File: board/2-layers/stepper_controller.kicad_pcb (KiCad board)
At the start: 4 copper layers, 99 x 46 mm, 126 parts, among them J201 USB_OTG, P101 JTAG, P102 JTAG, P103 CONN_4, P104 CONN_8X2, P105 CONN_4, P106 CONN_6X2, P107 CONN_4, P201 CONN_2X2, P301 12V_Conn, U101 DRV8825, U102 DRV8825, U103 DRV8825, U104 MAX5713/4/5-TSSOP14, U201 STM32F103RG_LQFP64, U301 MP2128-SOT23, U302 MP2303_SOIC8E, U401 XC3S200A, X201 TXC_50X32_AB

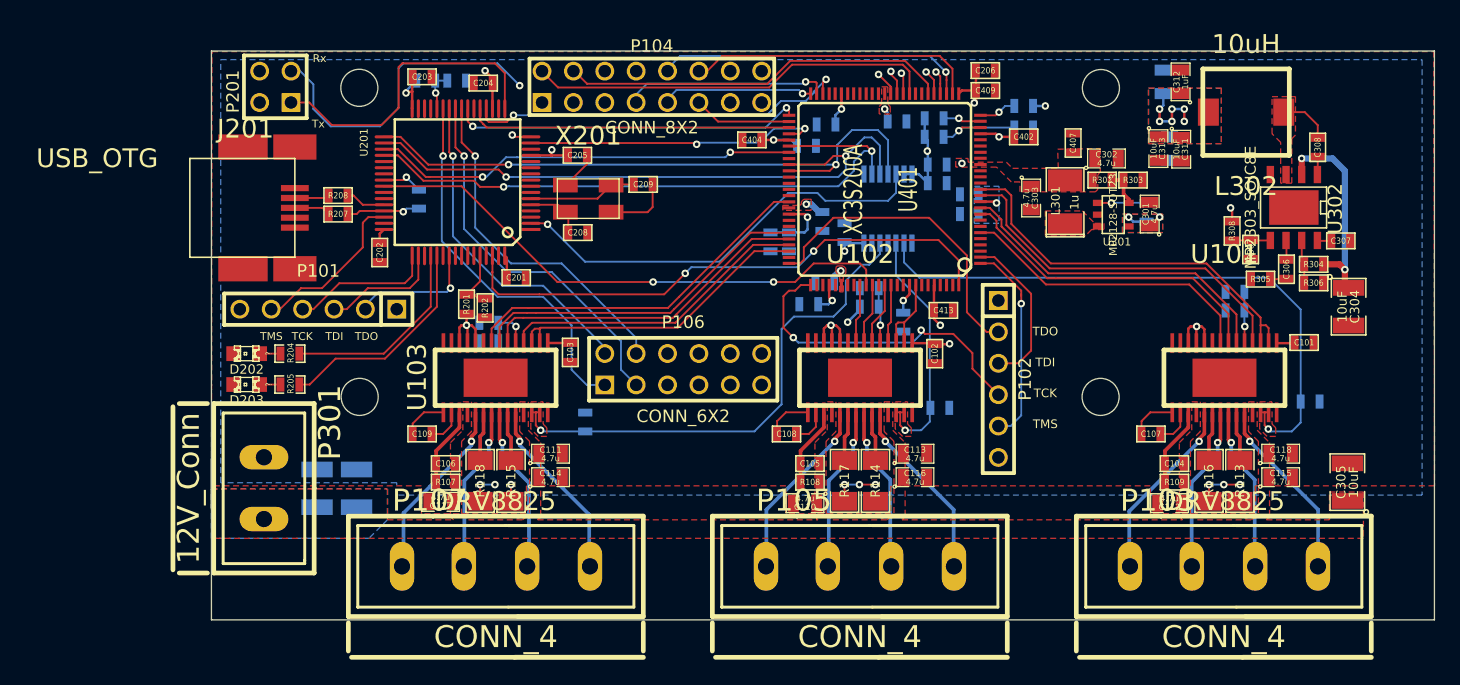
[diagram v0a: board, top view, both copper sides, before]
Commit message: pouet
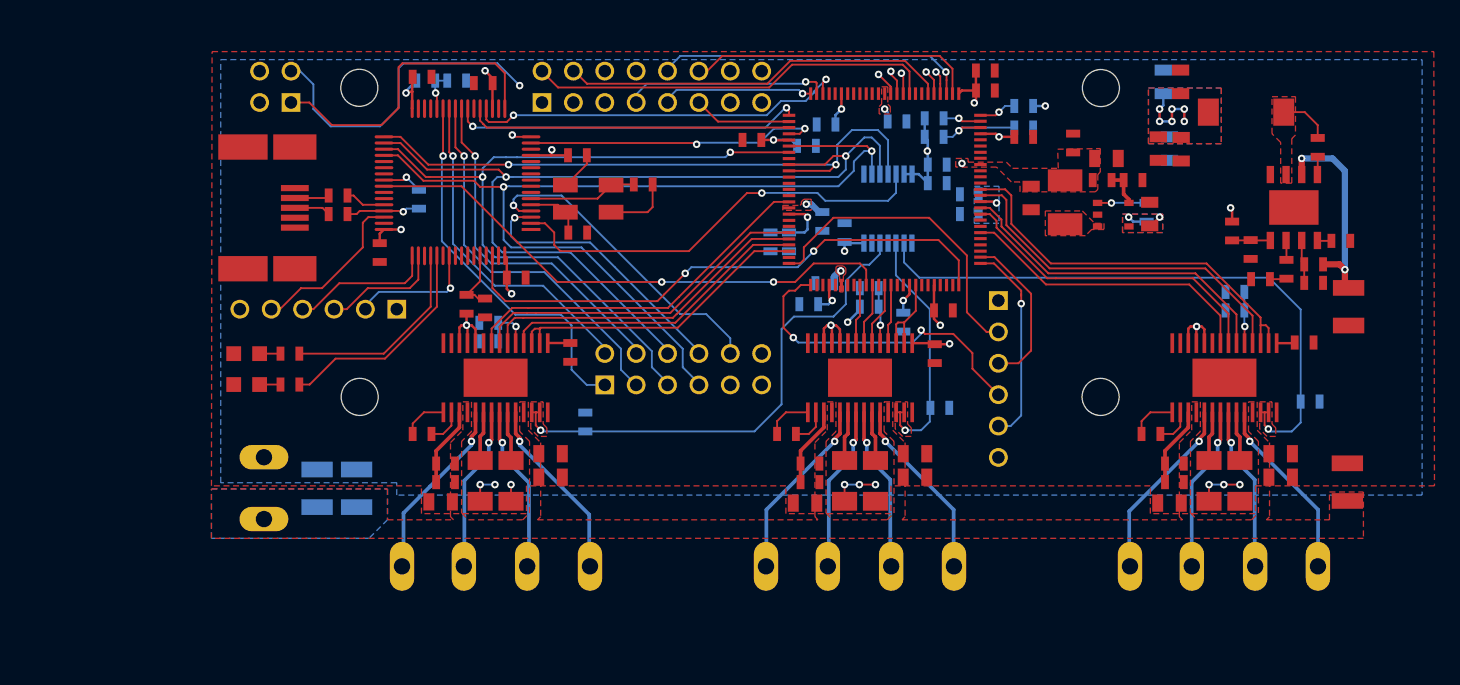
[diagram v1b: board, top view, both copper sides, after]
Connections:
- P106 pad 10: (no net) -> /STM32/PC15
- P106 pad 5: (no net) -> /FPGA/COM_MISO
- P106 pad 6: (no net) -> /FPGA/COM_CLK
- P106 pad 7: (no net) -> /FPGA/COM_MOSI
- P106 pad 8: (no net) -> /STM32/PC14
- U201 pad 3: (no net) -> /STM32/PC14
- U201 pad 4: (no net) -> /STM32/PC15
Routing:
- net /FPGA/COM_MISO: track 34.5 -> 61.0 mm
- net /FPGA/COM_MOSI: track 50.9 -> 76.8 mm
- net /STM32/PC15: track 0.00 -> 25.8 mm, vias 0 -> 1
- net /FPGA/COM_CLK: track 50.8 -> 75.1 mm
- net /STM32/PC14: track 0.00 -> 22.2 mm, vias 0 -> 1
- net +3.3V: track 90.2 -> 104.5 mm, vias 29 -> 31
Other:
- board outline removed
